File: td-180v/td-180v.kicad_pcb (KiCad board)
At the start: 2 copper layers, 73 x 28 mm, 21 parts, among them J18 Conn_01x02_Male, J2 Conn_01x02_Male, Q1 IPD50R3K0CE, U14 LT3758AEMSE

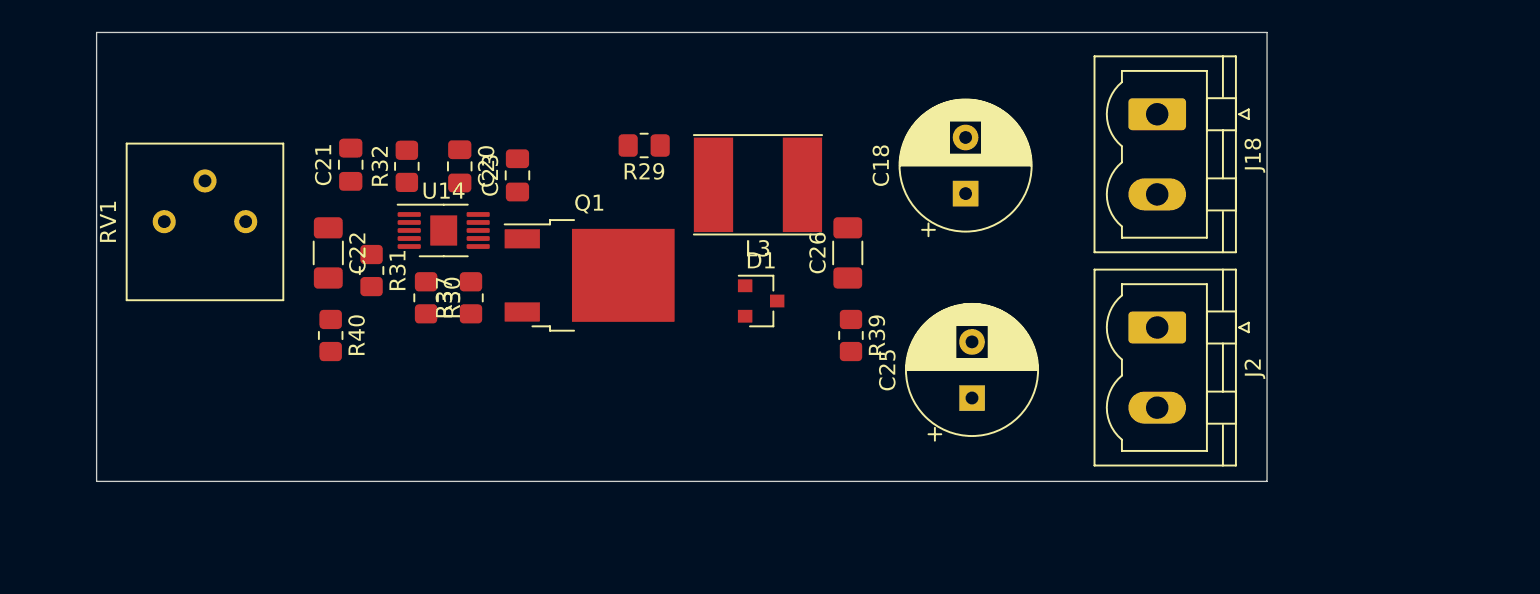
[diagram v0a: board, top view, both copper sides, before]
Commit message: 180v fixes
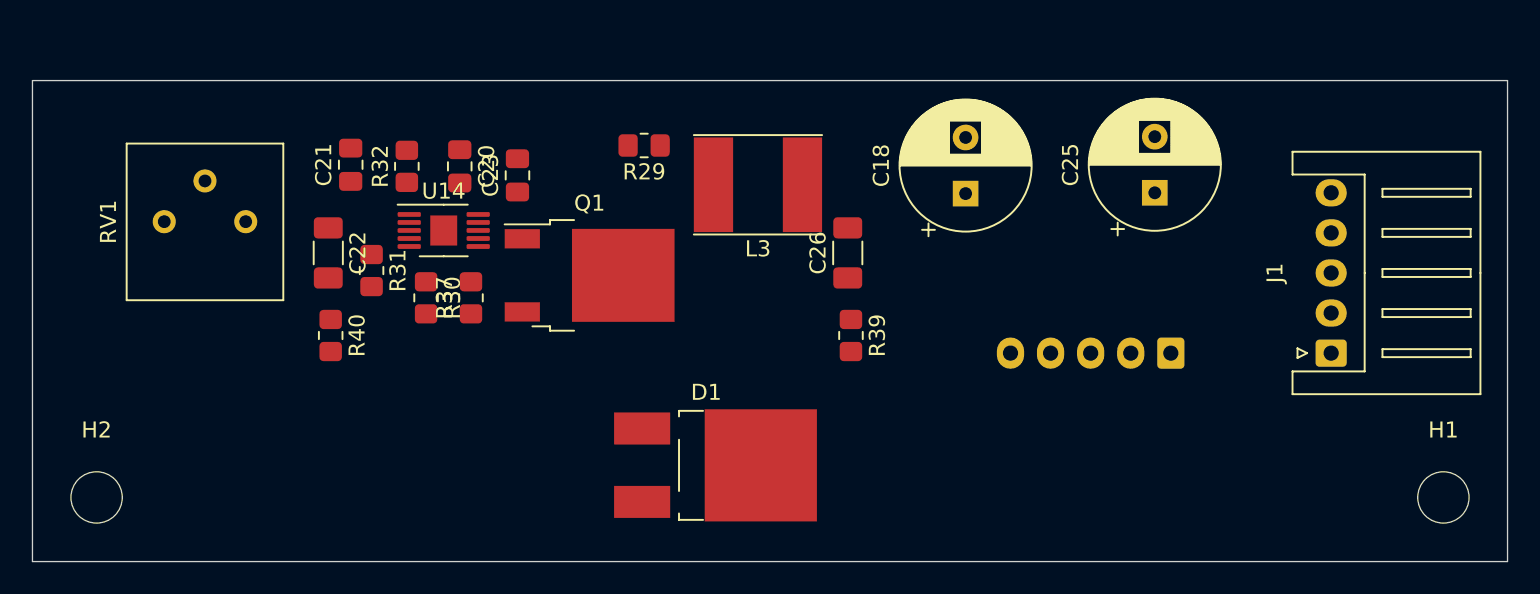
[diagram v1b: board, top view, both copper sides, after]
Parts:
- removed J18, J2: Conn_01x02_Male, Connector_Phoenix_MSTB:PhoenixContact_MSTBVA_2,5_2-G_1x02_P5.00mm_Vertical
- added H1: MountingHole, MountingHole:MountingHole_3.2mm_M3, F.Cu at (214.0, 130.0)
- added H2: MountingHole, MountingHole:MountingHole_3.2mm_M3, F.Cu at (130.0, 130.0)
- added J1: Conn_01x05_Male, Connector_JST:JST_XH_S5B-XH-A_1x05_P2.50mm_Horizontal, F.Cu at (207.0, 121.0)
- added J3: Conn_01x05_Male, Connector_JST:JST_XH_B5B-XH-A_1x05_P2.50mm_Vertical, B.Cu at (197.0, 121.0)
- D1: value BAS21 -> C3D02060E; footprint Package_TO_SOT_SMD:SOT-23 -> Package_TO_SOT_SMD:TO-252-2_TabPin1
- moved C25 17.1 mm to (196.0, 111.0)
- moved D1 10.6 mm to (168.6, 128.0)
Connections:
- D1 pad 1: Net-(D1-Pad1) -> HT
- L3 pad 2: Net-(D1-Pad1) -> Net-(D1-Pad2)
- Q1 pad 2: Net-(D1-Pad1) -> Net-(D1-Pad2)
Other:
- board size 73 x 28 mm -> 92 x 30 mm
